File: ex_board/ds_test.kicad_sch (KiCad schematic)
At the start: 67 parts, among them J2 DF40C-60DP-0.4V_51_, J3 Conn_01x30, J4 Conn_01x30

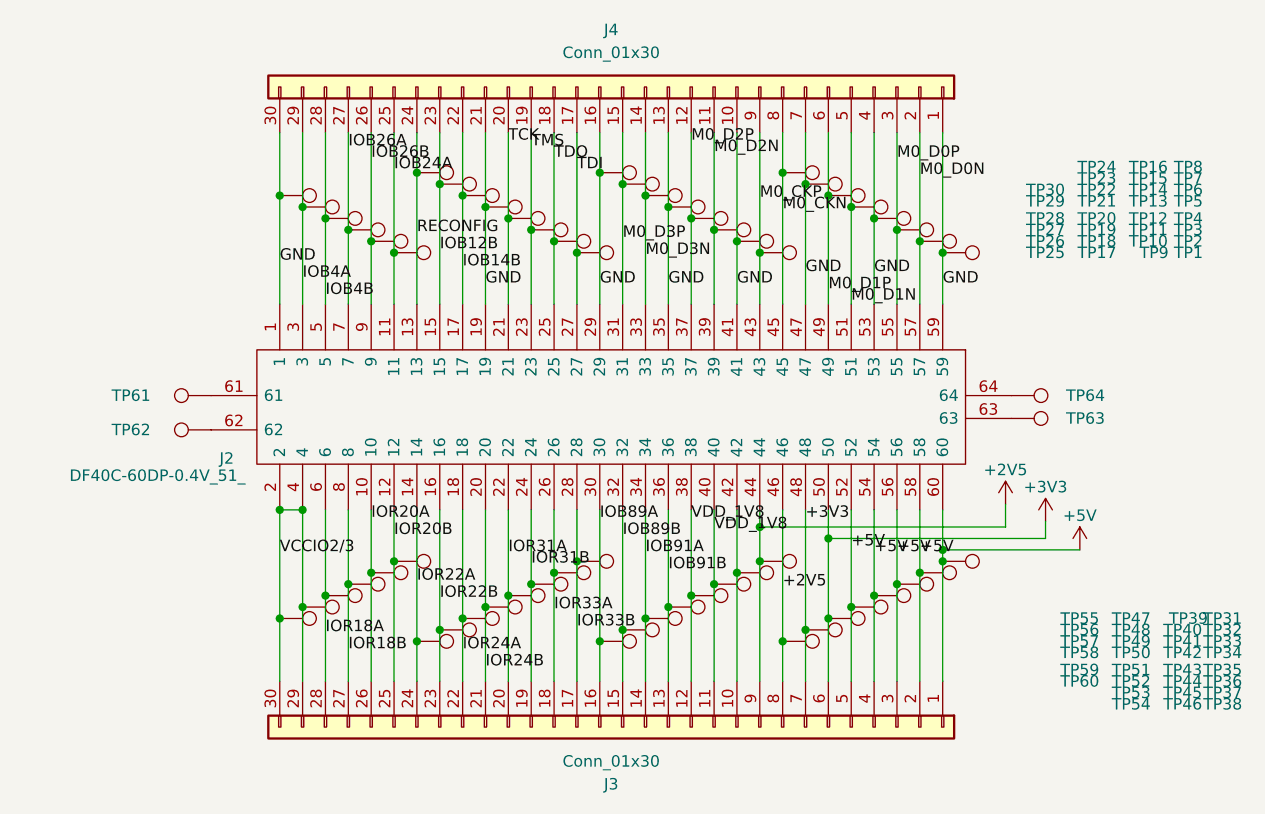
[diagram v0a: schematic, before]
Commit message: 1201
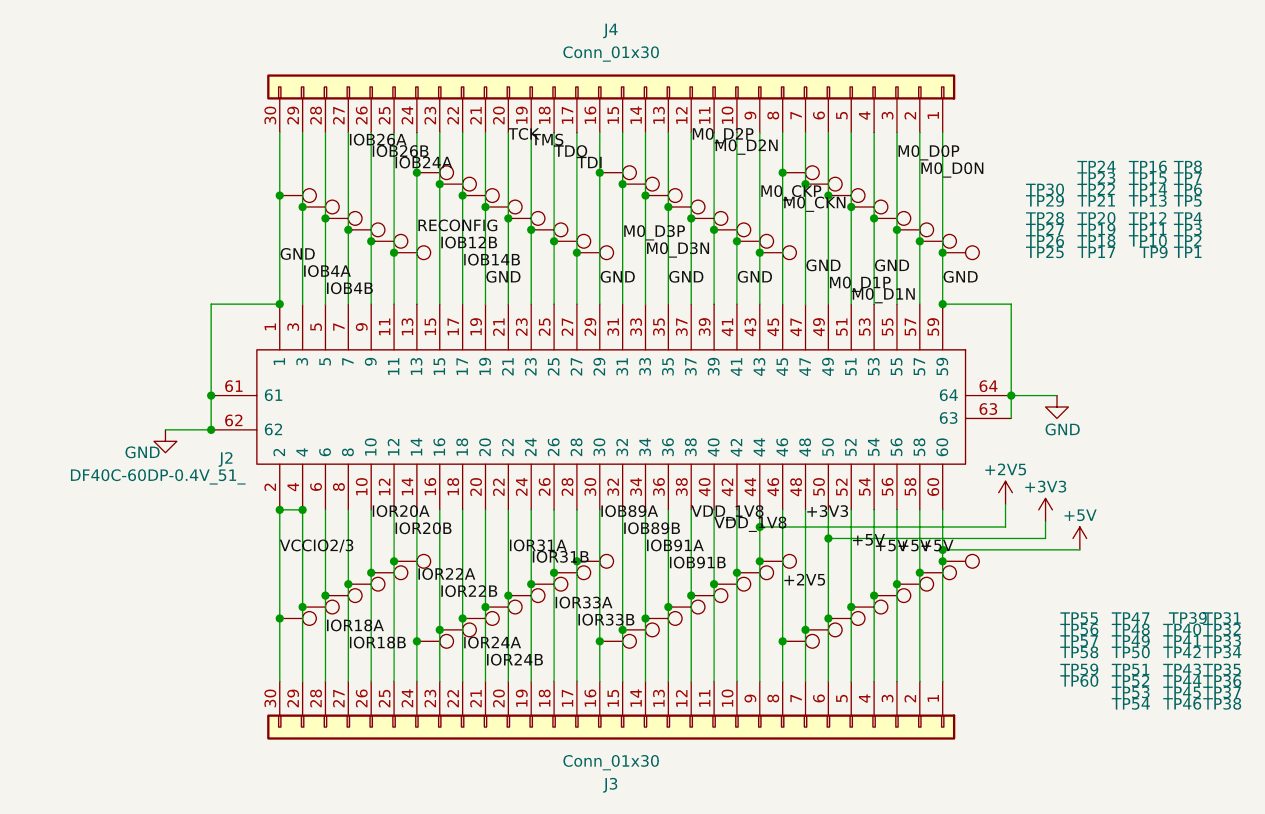
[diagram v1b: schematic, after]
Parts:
- removed TP61, TP62, TP63, TP64: TestPoint, TestPoint:TestPoint_Pad_1.5x1.5mm, symbol Connector:TestPoint
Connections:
- net GND: now also J2.61, J2.62, J2.63, J2.64
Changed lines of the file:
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@@
   (junction (at 66.675 95.885) (diameter 0) (color 0 0 0 0)
   )
+  (junction (at 59.055 74.93) (diameter 0) (color 0 0 0 0)
+  )
   (junction (at 127.635 48.895) (diameter 0) (color 0 0 0 0)
   )
@@
   (junction (at 132.715 93.345) (diameter 0) (color 0 0 0 0)
   )
+  (junction (at 59.055 71.12) (diameter 0) (color 0 0 0 0)
+  )
   (junction (at 107.315 48.895) (diameter 0) (color 0 0 0 0)
   )
@@
   (junction (at 125.095 97.155) (diameter 0) (color 0 0 0 0)
   )
+  (junction (at 66.675 60.96) (diameter 0) (color 0 0 0 0)
+  )
   (junction (at 71.755 51.435) (diameter 0) (color 0 0 0 0)
   )
@@
   (junction (at 89.535 94.615) (diameter 0) (color 0 0 0 0)
   )
+  (junction (at 140.335 60.96) (diameter 0) (color 0 0 0 0)
+  )
   (junction (at 99.695 55.245) (diameter 0) (color 0 0 0 0)
   )
@@
   (junction (at 125.095 47.625) (diameter 0) (color 0 0 0 0)
   )
+  (junction (at 147.955 71.12) (diameter 0) (color 0 0 0 0)
+  )
   (junction (at 127.635 86.995) (diameter 0) (color 0 0 0 0)
   )
@@
     (stroke (width 0) (type default))
   )
+  (wire (pts (xy 147.955 71.12) (xy 147.955 73.66))
+    (stroke (width 0) (type default))
+  )
   (wire (pts (xy 94.615 41.91) (xy 94.615 52.705))
     (stroke (width 0) (type default))
@@
     (stroke (width 0) (type default))
   )
+  (wire (pts (xy 140.335 60.96) (xy 147.955 60.96))
+    (stroke (width 0) (type default))
+  )
   (wire (pts (xy 94.615 83.82) (xy 94.615 92.075))
     (stroke (width 0) (type default))
@@
     (stroke (width 0) (type default))
   )
+  (wire (pts (xy 147.955 60.96) (xy 147.955 71.12))
+    (stroke (width 0) (type default))
+  )
   (wire (pts (xy 122.555 83.82) (xy 122.555 98.425))
     (stroke (width 0) (type default))
@@
     (stroke (width 0) (type default))
   )
+  (wire (pts (xy 59.055 71.12) (xy 59.055 74.93))
+    (stroke (width 0) (type default))
+  )
   (wire (pts (xy 79.375 41.91) (xy 79.375 55.245))
     (stroke (width 0) (type default))
@@
     (stroke (width 0) (type default))
   )
+  (wire (pts (xy 59.055 60.96) (xy 66.675 60.96))
+    (stroke (width 0) (type default))
+  )
   (wire (pts (xy 94.615 60.96) (xy 94.615 52.705))
     (stroke (width 0) (type default))
   )
+  (wire (pts (xy 147.955 71.12) (xy 153.035 71.12))
+    (stroke (width 0) (type default))
+  )
   (wire (pts (xy 86.995 83.82) (xy 86.995 95.885))
     (stroke (width 0) (type default))
@@
     (stroke (width 0) (type default))
   )
+  (wire (pts (xy 59.055 71.12) (xy 59.055 60.96))
+    (stroke (width 0) (type default))
+  )
   (wire (pts (xy 127.635 86.995) (xy 151.765 86.995))
     (stroke (width 0) (type default))
@@
     (stroke (width 0) (type default))
   )
+  (wire (pts (xy 53.975 74.93) (xy 59.055 74.93))
+    (stroke (width 0) (type default))
+  )
   (wire (pts (xy 89.535 83.82) (xy 89.535 94.615))
     (stroke (width 0) (type default))
@@
     )
   )
+  (symbol (lib_id "power:GND") (at 53.975 74.93 0) (unit 1)
+    (in_bom yes) (on_board yes) (dnp no)
+    (property "Reference" "#PWR01" (at 53.975 81.28 0)
+      (effects (font (size 1.27 1.27)) hide)
+    )
+    (property "Value" "GND" (at 51.435 77.47 0)
+      (effects (font (size 1.27 1.27)))
+    )
+    (property "Footprint" "" (at 53.975 74.93 0)
+      (effects (font (size 1.27 1.27)) hide)
+    )
+    (property "Datasheet" "" (at 53.975 74.93 0)
+      (effects (font (size 1.27 1.27)) hide)
+    )
+    (pin "1")
+    (instances
+      (project "ds_test"
+        (path "/39a416e3-9027-4b62-bcd6-affd237dabf1"
+          (reference "#PWR01") (unit 1)
+        )
+      )
+    )
+  )
   (symbol (lib_id "Connector:TestPoint") (at 127.635 95.885 270) (mirror x) (unit 1)
     (in_bom yes) (on_board yes) (dnp no)
@@
         (path "/39a416e3-9027-4b62-bcd6-affd237dabf1"
           (reference "TP60") (unit 1)
-        )
-      )
-    )
-  )
-  (symbol (lib_id "Connector:TestPoint") (at 59.055 74.93 90) (unit 1)
-    (in_bom yes) (on_board yes) (dnp no)
-    (property "Reference" "TP62" (at 50.165 74.93 90)
-      (effects (font (size 1.27 1.27)))
-    )
-    (property "Value" "TestPoint" (at 55.753 71.755 90)
-      (effects (font (size 1.27 1.27)) hide)
-    )
-    (property "Footprint" "TestPoint:TestPoint_Pad_1.5x1.5mm" (at 59.055 69.85 0)
-      (effects (font (size 1.27 1.27)) hide)
-    )
-    (property "Datasheet" "~" (at 59.055 69.85 0)
-      (effects (font (size 1.27 1.27)) hide)
-    )
-    (pin "1")
-    (instances
-      (project "ds_test"
-        (path "/39a416e3-9027-4b62-bcd6-affd237dabf1"
-          (reference "TP62") (unit 1)
         )
       )
@@
     )
   )
-  (symbol (lib_id "Connector:TestPoint") (at 59.055 71.12 90) (unit 1)
-    (in_bom yes) (on_board yes) (dnp no)
-    (property "Reference" "TP61" (at 50.165 71.12 90)
-      (effects (font (size 1.27 1.27)))
-    )
-    (property "Value" "TestPoint" (at 55.753 67.945 90)
-      (effects (font (size 1.27 1.27)) hide)
-    )
-    (property "Footprint" "TestPoint:TestPoint_Pad_1.5x1.5mm" (at 59.055 66.04 0)
-      (effects (font (size 1.27 1.27)) hide)
-    )
-    (property "Datasheet" "~" (at 59.055 66.04 0)
-      (effects (font (size 1.27 1.27)) hide)
-    )
-    (pin "1")
-    (instances
-      (project "ds_test"
-        (path "/39a416e3-9027-4b62-bcd6-affd237dabf1"
-          (reference "TP61") (unit 1)
-        )
-      )
-    )
-  )
-  (symbol (lib_id "Connector:TestPoint") (at 147.955 73.66 270) (unit 1)
-    (in_bom yes) (on_board yes) (dnp no)
-    (property "Reference" "TP63" (at 156.21 73.66 90)
-      (effects (font (size 1.27 1.27)))
-    )
-    (property "Value" "TestPoint" (at 151.257 76.835 90)
-      (effects (font (size 1.27 1.27)) hide)
-    )
-    (property "Footprint" "TestPoint:TestPoint_Pad_1.5x1.5mm" (at 147.955 78.74 0)
-      (effects (font (size 1.27 1.27)) hide)
-    )
-    (property "Datasheet" "~" (at 147.955 78.74 0)
-      (effects (font (size 1.27 1.27)) hide)
-    )
-    (pin "1")
-    (instances
-      (project "ds_test"
-        (path "/39a416e3-9027-4b62-bcd6-affd237dabf1"
-          (reference "TP63") (unit 1)
-        )
-      )
-    )
-  )
-  (symbol (lib_id "Connector:TestPoint") (at 147.955 71.12 270) (unit 1)
-    (in_bom yes) (on_board yes) (dnp no)
-    (property "Reference" "TP64" (at 156.21 71.12 90)
-      (effects (font (size 1.27 1.27)))
-    )
-    (property "Value" "TestPoint" (at 151.257 74.295 90)
-      (effects (font (size 1.27 1.27)) hide)
-    )
-    (property "Footprint" "TestPoint:TestPoint_Pad_1.5x1.5mm" (at 147.955 76.2 0)
-      (effects (font (size 1.27 1.27)) hide)
-    )
-    (property "Datasheet" "~" (at 147.955 76.2 0)
-      (effects (font (size 1.27 1.27)) hide)
-    )
-    (pin "1")
-    (instances
-      (project "ds_test"
-        (path "/39a416e3-9027-4b62-bcd6-affd237dabf1"
-          (reference "TP64") (unit 1)
-        )
-      )
+  (symbol (lib_id "power:GND") (at 153.035 71.12 0) (unit 1)
+    (in_bom yes) (on_board yes) (dnp no)
+    (property "Reference" "#PWR02" (at 153.035 77.47 0)
+      (effects (font (size 1.27 1.27)) hide)
+    )
+    (property "Value" "GND" (at 153.67 74.93 0)
+      (effects (font (size 1.27 1.27)))
+    )
+    (property "Footprint" "" (at 153.035 71.12 0)
+      (effects (font (size 1.27 1.27)) hide)
+    )
+    (property "Datasheet" "" (at 153.035 71.12 0)
+      (effects (font (size 1.27 1.27)) hide)
+    )
+    (pin "1")
+    (instances
+      (project "ds_test"
+        (path "/39a416e3-9027-4b62-bcd6-affd237dabf1"
+          (reference "#PWR02") (unit 1)
+        )
+      )
